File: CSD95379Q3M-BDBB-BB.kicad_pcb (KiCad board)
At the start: 4 copper layers, 48 x 30 mm, 23 parts, among them U101 CSD97394Q4M, U102 CSD97394Q4M, U103 INA260, U104 INA260

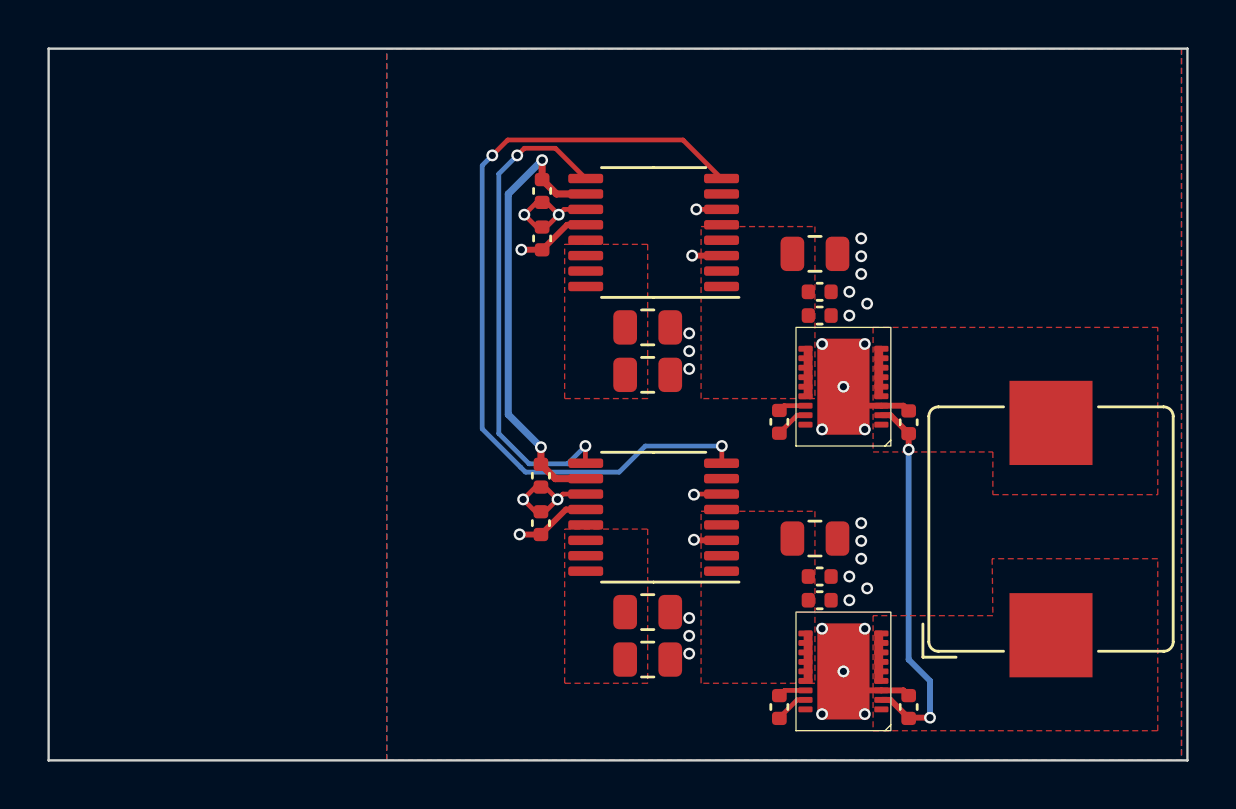
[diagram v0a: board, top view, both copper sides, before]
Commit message: Route some more stuff, move things a bit.
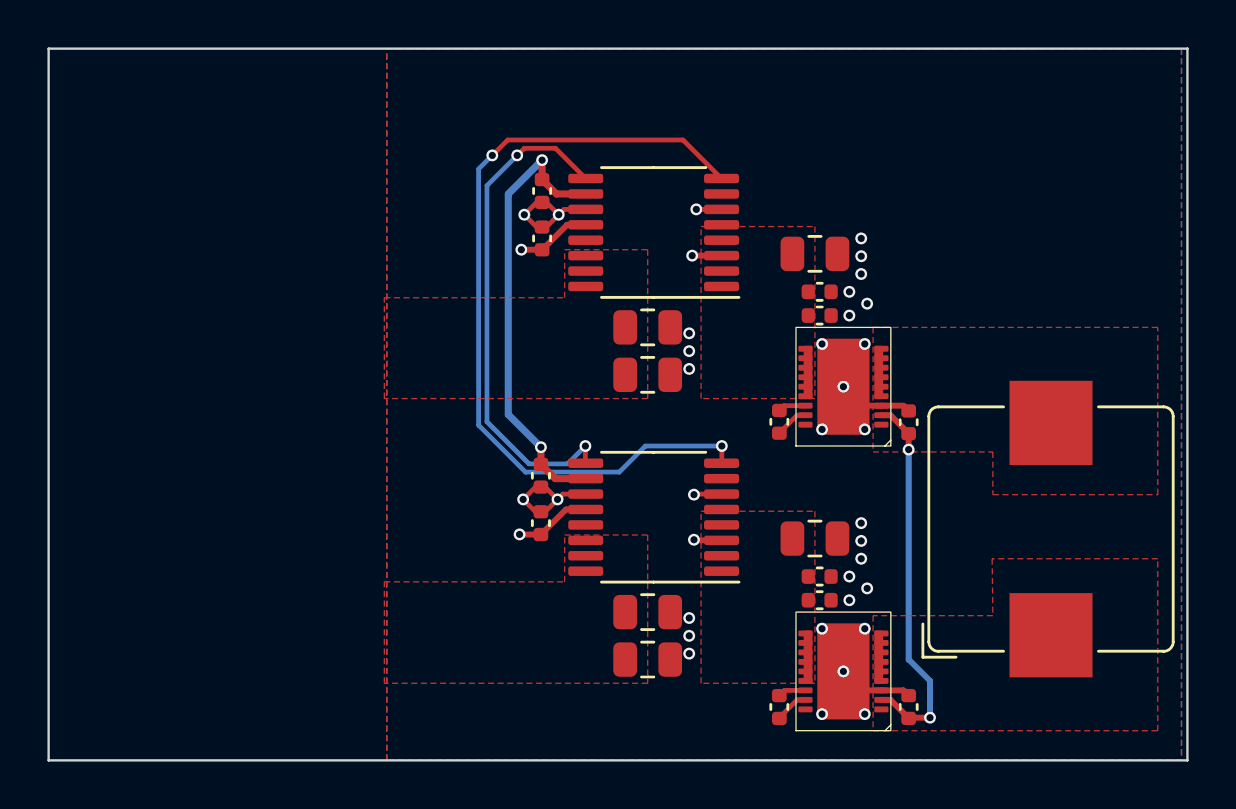
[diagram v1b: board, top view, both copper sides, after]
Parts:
- C113, C115: value .1uF X5R 35V -> .1uF X7S 10V
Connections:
- net /VSWA renamed Net-(U101-VSW)
- U101 pad 1: unconnected-(U101-~{SKIP}-Pad1) -> /~{SKIP}-A
- U101 pad 8: unconnected-(U101-PWM-Pad8) -> /PWM-A
- U102 pad 1: unconnected-(U102-~{SKIP}-Pad1) -> /~{SKIP}-B
- U102 pad 8: unconnected-(U102-PWM-Pad8) -> /PWM-B
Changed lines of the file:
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@@
   )
   (net 0 "")
-  (net 1 "unconnected-(U101-~{SKIP}-Pad1)")
-  (net 2 "unconnected-(U102-~{SKIP}-Pad1)")
+  (net 1 "Net-(U101-VSW)")
+  (net 2 "/~{SKIP}-A")
   (net 3 "Net-(U101-BOOT)")
   (net 4 "Net-(U101-BOOT_R)")
@@
   (net 8 "/VA")
   (net 9 "/VB")
-  (net 10 "/VSWA")
+  (net 10 "/PWM-A")
   (net 11 "/VSWB")
   (net 12 "+5V")
-  (net 13 "unconnected-(U101-PWM-Pad8)")
-  (net 14 "unconnected-(U102-PWM-Pad8)")
+  (net 13 "/~{SKIP}-B")
+  (net 14 "/PWM-B")
   (net 15 "unconnected-(U103-A1-Pad4)")
   (net 16 "unconnected-(U103-A0-Pad5)")
@@
         (effects (font (size 1 1) (thickness 0.15)))
     )
-    (fp_text value ".1uF X5R 35V" (at 0 1.16 90) (layer "F.Fab") hide
+    (fp_text value ".1uF X7S 10V" (at 0 1.16 90) (layer "F.Fab") hide
         (effects (font (size 1 1) (thickness 0.15)))
     )
@@
         (effects (font (size 1 1) (thickness 0.15)))
     )
-    (fp_text value ".1uF X5R 35V" (at 0 1.16 90) (layer "F.Fab") hide
+    (fp_text value ".1uF X7S 10V" (at 0 1.16 90) (layer "F.Fab") hide
         (effects (font (size 1 1) (thickness 0.15)))
     )
@@
       (stroke (width 0.05) (type default)) (fill none) (layer "F.Fab"))
     (pad "1" smd roundrect (at -1.6 1.6 90) (size 0.25 0.6) (layers "F.Cu" "F.Paste" "F.Mask") (roundrect_rratio 0.2)
-      (net 1 "unconnected-(U101-~{SKIP}-Pad1)") (pinfunction "~{SKIP}") (pintype "input") (thermal_bridge_angle 45))
+      (net 2 "/~{SKIP}-A") (pinfunction "~{SKIP}") (pintype "input") (thermal_bridge_angle 45))
     (pad "2" smd roundrect (at -1.2 1.6 90) (size 0.25 0.6) (layers "F.Cu" "F.Paste" "F.Mask") (roundrect_rratio 0.2)
       (net 12 "+5V") (pinfunction "VDD") (pintype "power_in") (thermal_bridge_angle 45))
@@
       (net 7 "GND") (pinfunction "PGND") (pintype "power_in") (thermal_bridge_angle 45))
     (pad "4" smd roundrect (at -0.4 1.6 90) (size 0.25 0.6) (layers "F.Cu" "F.Paste" "F.Mask") (roundrect_rratio 0.2)
-      (net 10 "/VSWA") (pinfunction "VSW") (pintype "power_out") (thermal_bridge_angle 45))
+      (net 1 "Net-(U101-VSW)") (pinfunction "VSW") (pintype "power_out") (thermal_bridge_angle 45))
     (pad "4" smd roundrect (at 0 1.6 90) (size 0.25 0.6) (layers "F.Cu" "F.Paste" "F.Mask") (roundrect_rratio 0.2)
-      (net 10 "/VSWA") (pinfunction "VSW") (pintype "power_out") (thermal_bridge_angle 45))
+      (net 1 "Net-(U101-VSW)") (pinfunction "VSW") (pintype "power_out") (thermal_bridge_angle 45))
     (pad "4" smd roundrect (at 0.4 1.6 90) (size 0.25 0.6) (layers "F.Cu" "F.Paste" "F.Mask") (roundrect_rratio 0.2)
-      (net 10 "/VSWA") (pinfunction "VSW") (pintype "power_out") (thermal_bridge_angle 45))
+      (net 1 "Net-(U101-VSW)") (pinfunction "VSW") (pintype "power_out") (thermal_bridge_angle 45))
     (pad "4" smd roundrect (at 0.6 1.49 90) (size 2.25 0.375) (layers "F.Cu" "F.Paste" "F.Mask") (roundrect_rratio 0.1692053333)
-      (net 10 "/VSWA") (pinfunction "VSW") (pintype "power_out") (thermal_bridge_angle 45))
+      (net 1 "Net-(U101-VSW)") (pinfunction "VSW") (pintype "power_out") (thermal_bridge_angle 45))
     (pad "4" smd roundrect (at 0.8 1.6 90) (size 0.25 0.6) (layers "F.Cu" "F.Paste" "F.Mask") (roundrect_rratio 0.2)
-      (net 10 "/VSWA") (pinfunction "VSW") (pintype "power_out") (thermal_bridge_angle 45))
+      (net 1 "Net-(U101-VSW)") (pinfunction "VSW") (pintype "power_out") (thermal_bridge_angle 45))
     (pad "4" smd roundrect (at 1.2 1.6 90) (size 0.25 0.6) (layers "F.Cu" "F.Paste" "F.Mask") (roundrect_rratio 0.2)
-      (net 10 "/VSWA") (pinfunction "VSW") (pintype "power_out") (thermal_bridge_angle 45))
+      (net 1 "Net-(U101-VSW)") (pinfunction "VSW") (pintype "power_out") (thermal_bridge_angle 45))
     (pad "4" smd roundrect (at 1.6 1.6 90) (size 0.25 0.6) (layers "F.Cu" "F.Paste" "F.Mask") (roundrect_rratio 0.2)
-      (net 10 "/VSWA") (pinfunction "VSW") (pintype "power_out") (thermal_bridge_angle 45))
+      (net 1 "Net-(U101-VSW)") (pinfunction "VSW") (pintype "power_out") (thermal_bridge_angle 45))
     (pad "5" smd roundrect (at -0.4 -1.6 90) (size 0.25 0.6) (layers "F.Cu" "F.Paste" "F.Mask") (roundrect_rratio 0.2)
       (net 19 "/VAS") (pinfunction "VIN") (pintype "power_in") (thermal_bridge_angle 45))
@@
       (net 3 "Net-(U101-BOOT)") (pinfunction "BOOT") (pintype "passive") (thermal_bridge_angle 45))
     (pad "8" smd roundrect (at -1.6 -1.6 90) (size 0.25 0.6) (layers "F.Cu" "F.Paste" "F.Mask") (roundrect_rratio 0.2)
-      (net 13 "unconnected-(U101-PWM-Pad8)") (pinfunction "PWM") (pintype "input") (thermal_bridge_angle 45))
+      (net 10 "/PWM-A") (pinfunction "PWM") (pintype "input") (thermal_bridge_angle 45))
     (pad "9" smd roundrect (at 0 0 90) (size 4.05 2.2) (layers "F.Cu" "F.Paste" "F.Mask") (roundrect_rratio 0.04545454545)
       (net 7 "GND") (pinfunction "PGND") (pintype "power_in") (thermal_bridge_angle 45))
@@
       (stroke (width 0.1) (type solid)) (layer "F.Fab"))
     (pad "1" smd rect (at -4.475 0 90) (size 3.55 3.5) (layers "F.Cu" "F.Paste" "F.Mask")
-      (net 10 "/VSWA") (pinfunction "1") (pintype "passive"))
+      (net 1 "Net-(U101-VSW)") (pinfunction "1") (pintype "passive"))
     (pad "2" smd rect (at 4.475 0 90) (size 3.55 3.5) (layers "F.Cu" "F.Paste" "F.Mask")
       (net 11 "/VSWB") (pinfunction "2") (pintype "passive"))
@@
       (stroke (width 0.05) (type default)) (fill none) (layer "F.Fab"))
     (pad "1" smd roundrect (at -1.6 1.6 90) (size 0.25 0.6) (layers "F.Cu" "F.Paste" "F.Mask") (roundrect_rratio 0.2)
-      (net 2 "unconnected-(U102-~{SKIP}-Pad1)") (pinfunction "~{SKIP}") (pintype "input") (thermal_bridge_angle 45))
+      (net 13 "/~{SKIP}-B") (pinfunction "~{SKIP}") (pintype "input") (thermal_bridge_angle 45))
     (pad "2" smd roundrect (at -1.2 1.6 90) (size 0.25 0.6) (layers "F.Cu" "F.Paste" "F.Mask") (roundrect_rratio 0.2)
       (net 12 "+5V") (pinfunction "VDD") (pintype "power_in") (thermal_bridge_angle 45))
@@
       (net 6 "Net-(U102-BOOT)") (pinfunction "BOOT") (pintype "passive") (thermal_bridge_angle 45))
     (pad "8" smd roundrect (at -1.6 -1.6 90) (size 0.25 0.6) (layers "F.Cu" "F.Paste" "F.Mask") (roundrect_rratio 0.2)
-      (net 14 "unconnected-(U102-PWM-Pad8)") (pinfunction "PWM") (pintype "input") (thermal_bridge_angle 45))
+      (net 14 "/PWM-B") (pinfunction "PWM") (pintype "input") (thermal_bridge_angle 45))
     (pad "9" smd roundrect (at 0 0 90) (size 4.05 2.2) (layers "F.Cu" "F.Paste" "F.Mask") (roundrect_rratio 0.04545454545)
       (net 7 "GND") (pinfunction "PGND") (pintype "power_in") (thermal_bridge_angle 45))
@@
   (via (at 152.875 113.5) (size 0.5) (drill 0.3) (layers "F.Cu" "B.Cu") (net 26))
   (via (at 143.2 101.25) (size 0.5) (drill 0.3) (layers "F.Cu" "B.Cu") (net 26))
+  (segment (start 144.6 114.6) (end 148.55 114.6) (width 0.2) (layer "B.Cu") (net 26))
+  (segment (start 142.625 101.825) (end 142.625 112.625) (width 0.2) (layer "B.Cu") (net 26))
   (segment (start 149.65 113.5) (end 152.875 113.5) (width 0.2) (layer "B.Cu") (net 26))
-  (segment (start 144.4 114.4) (end 144.6 114.6) (width 0.2) (layer "B.Cu") (net 26))
-  (segment (start 143.2 101.25) (end 142.775 101.675) (width 0.2) (layer "B.Cu") (net 26))
-  (segment (start 142.775 101.675) (end 142.775 112.775) (width 0.2) (layer "B.Cu") (net 26))
-  (segment (start 144.6 114.6) (end 148.55 114.6) (width 0.2) (layer "B.Cu") (net 26))
+  (segment (start 142.625 112.625) (end 144.6 114.6) (width 0.2) (layer "B.Cu") (net 26))
   (segment (start 148.55 114.6) (end 149.65 113.5) (width 0.2) (layer "B.Cu") (net 26))
-  (segment (start 142.775 112.775) (end 144.4 114.4) (width 0.2) (layer "B.Cu") (net 26))
+  (segment (start 143.2 101.25) (end 142.625 101.825) (width 0.2) (layer "B.Cu") (net 26))
   (segment (start 147.125 114.2125) (end 147.1375 114.225) (width 0.2) (layer "F.Cu") (net 27))
   (segment (start 147.1375 102.225) (end 145.8625 100.95) (width 0.2) (layer "F.Cu") (net 27))
@@
   (via (at 144.25 101.25) (size 0.5) (drill 0.3) (layers "F.Cu" "B.Cu") (net 27))
   (via (at 147.125 113.5) (size 0.5) (drill 0.3) (layers "F.Cu" "B.Cu") (net 27))
+  (segment (start 142.975 112.475) (end 144.75 114.25) (width 0.2) (layer "B.Cu") (net 27))
+  (segment (start 146.375 114.25) (end 147.125 113.5) (width 0.2) (layer "B.Cu") (net 27))
+  (segment (start 144.25 101.25) (end 142.975 102.525) (width 0.2) (layer "B.Cu") (net 27))
+  (segment (start 142.975 102.525) (end 142.975 112.475) (width 0.2) (layer "B.Cu") (net 27))
   (segment (start 144.75 114.25) (end 146.375 114.25) (width 0.2) (layer "B.Cu") (net 27))
-  (segment (start 144.25 101.25) (end 143.475 102.025) (width 0.2) (layer "B.Cu") (net 27))
-  (segment (start 146.375 114.25) (end 147.125 113.5) (width 0.2) (layer "B.Cu") (net 27))
-  (segment (start 143.475 112.975) (end 144.75 114.25) (width 0.2) (layer "B.Cu") (net 27))
-  (segment (start 143.475 102.025) (end 143.475 112.975) (width 0.2) (layer "B.Cu") (net 27))
   (zone (net 11) (net_name "/VSWB") (layer "F.Cu") (hatch edge 0.5)
     (priority 1)
@@
     )
   )
-  (zone (net 10) (net_name "/VSWA") (layer "F.Cu") (hatch edge 0.5)
+  (zone (net 1) (net_name "Net-(U101-VSW)") (layer "F.Cu") (hatch edge 0.5)
     (connect_pads yes (clearance 0.25))
     (min_thickness 0.25) (filled_areas_thickness no)
@@
     (polygon
       (pts
-        (xy 146.25 105)
-        (xy 149.75 105)
+        (xy 138.648856 107.25)
+        (xy 146.25 107.25)
+        (xy 146.25 105.225)
+        (xy 149.75 105.225)
         (xy 149.75 111.5)
-        (xy 146.25 111.5)
+        (xy 138.65 111.5)
       )
     )
@@
     (polygon
       (pts
-        (xy 146.25 117)
-        (xy 149.75 117)
+        (xy 138.65 119.225)
+        (xy 146.25 119.225)
+        (xy 146.25 117.25)
+        (xy 149.75 117.25)
         (xy 149.75 123.5)
-        (xy 146.25 123.5)
+        (xy 138.65 123.5)
       )
     )

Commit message: Fixed a net name.
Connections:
- net Net-(U101-VSW) renamed /VSWA
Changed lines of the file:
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@@
   )
   (net 0 "")
-  (net 1 "Net-(U101-VSW)")
+  (net 1 "/VSWA")
   (net 2 "/~{SKIP}-A")
   (net 3 "Net-(U101-BOOT)")
@@
       (net 7 "GND") (pinfunction "PGND") (pintype "power_in") (thermal_bridge_angle 45))
     (pad "4" smd roundrect (at -0.4 1.6 90) (size 0.25 0.6) (layers "F.Cu" "F.Paste" "F.Mask") (roundrect_rratio 0.2)
-      (net 1 "Net-(U101-VSW)") (pinfunction "VSW") (pintype "power_out") (thermal_bridge_angle 45))
+      (net 1 "/VSWA") (pinfunction "VSW") (pintype "power_out") (thermal_bridge_angle 45))
     (pad "4" smd roundrect (at 0 1.6 90) (size 0.25 0.6) (layers "F.Cu" "F.Paste" "F.Mask") (roundrect_rratio 0.2)
-      (net 1 "Net-(U101-VSW)") (pinfunction "VSW") (pintype "power_out") (thermal_bridge_angle 45))
+      (net 1 "/VSWA") (pinfunction "VSW") (pintype "power_out") (thermal_bridge_angle 45))
     (pad "4" smd roundrect (at 0.4 1.6 90) (size 0.25 0.6) (layers "F.Cu" "F.Paste" "F.Mask") (roundrect_rratio 0.2)
-      (net 1 "Net-(U101-VSW)") (pinfunction "VSW") (pintype "power_out") (thermal_bridge_angle 45))
+      (net 1 "/VSWA") (pinfunction "VSW") (pintype "power_out") (thermal_bridge_angle 45))
     (pad "4" smd roundrect (at 0.6 1.49 90) (size 2.25 0.375) (layers "F.Cu" "F.Paste" "F.Mask") (roundrect_rratio 0.1692053333)
-      (net 1 "Net-(U101-VSW)") (pinfunction "VSW") (pintype "power_out") (thermal_bridge_angle 45))
+      (net 1 "/VSWA") (pinfunction "VSW") (pintype "power_out") (thermal_bridge_angle 45))
     (pad "4" smd roundrect (at 0.8 1.6 90) (size 0.25 0.6) (layers "F.Cu" "F.Paste" "F.Mask") (roundrect_rratio 0.2)
-      (net 1 "Net-(U101-VSW)") (pinfunction "VSW") (pintype "power_out") (thermal_bridge_angle 45))
+      (net 1 "/VSWA") (pinfunction "VSW") (pintype "power_out") (thermal_bridge_angle 45))
     (pad "4" smd roundrect (at 1.2 1.6 90) (size 0.25 0.6) (layers "F.Cu" "F.Paste" "F.Mask") (roundrect_rratio 0.2)
-      (net 1 "Net-(U101-VSW)") (pinfunction "VSW") (pintype "power_out") (thermal_bridge_angle 45))
+      (net 1 "/VSWA") (pinfunction "VSW") (pintype "power_out") (thermal_bridge_angle 45))
     (pad "4" smd roundrect (at 1.6 1.6 90) (size 0.25 0.6) (layers "F.Cu" "F.Paste" "F.Mask") (roundrect_rratio 0.2)
-      (net 1 "Net-(U101-VSW)") (pinfunction "VSW") (pintype "power_out") (thermal_bridge_angle 45))
+      (net 1 "/VSWA") (pinfunction "VSW") (pintype "power_out") (thermal_bridge_angle 45))
     (pad "5" smd roundrect (at -0.4 -1.6 90) (size 0.25 0.6) (layers "F.Cu" "F.Paste" "F.Mask") (roundrect_rratio 0.2)
       (net 19 "/VAS") (pinfunction "VIN") (pintype "power_in") (thermal_bridge_angle 45))
@@
       (stroke (width 0.1) (type solid)) (layer "F.Fab"))
     (pad "1" smd rect (at -4.475 0 90) (size 3.55 3.5) (layers "F.Cu" "F.Paste" "F.Mask")
-      (net 1 "Net-(U101-VSW)") (pinfunction "1") (pintype "passive"))
+      (net 1 "/VSWA") (pinfunction "1") (pintype "passive"))
     (pad "2" smd rect (at 4.475 0 90) (size 3.55 3.5) (layers "F.Cu" "F.Paste" "F.Mask")
       (net 11 "/VSWB") (pinfunction "2") (pintype "passive"))
@@
     )
   )
-  (zone (net 1) (net_name "Net-(U101-VSW)") (layer "F.Cu") (hatch edge 0.5)
+  (zone (net 1) (net_name "/VSWA") (layer "F.Cu") (hatch edge 0.5)
     (connect_pads yes (clearance 0.25))
     (min_thickness 0.25) (filled_areas_thickness no)
